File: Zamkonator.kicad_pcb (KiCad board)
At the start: 2 copper layers, 75 x 75 mm, 104 parts, among them J1 Screw_Terminal_01x06, J2 RJ45_Abracon_ARJP11A-MASA-B-A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, J3 Conn_01x08_Male, J4 Conn_02x08_Counter_Clockwise, K1 SRD-DC3V-SL-C, Q1 BCP56, T1 HR051142, U1 RTL8201F, U2 SI3404-A-GM, U3 EL3H7-G, U4 AN431, U5 MT2492, U6 ESP32-WROOM-32, U7 LTV-827S, U8 LTV-827S, X1 S3D50.000000B20F30T

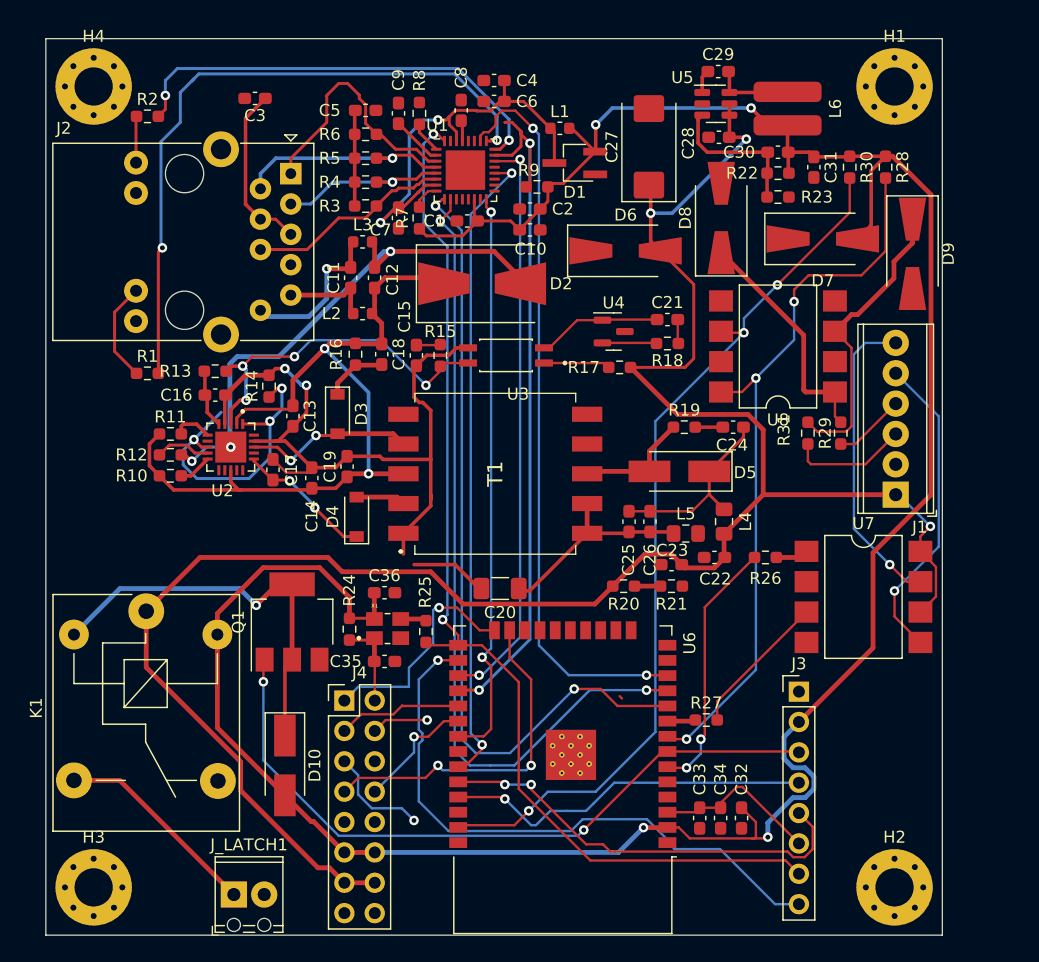
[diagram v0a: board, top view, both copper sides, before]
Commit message: Finish layout
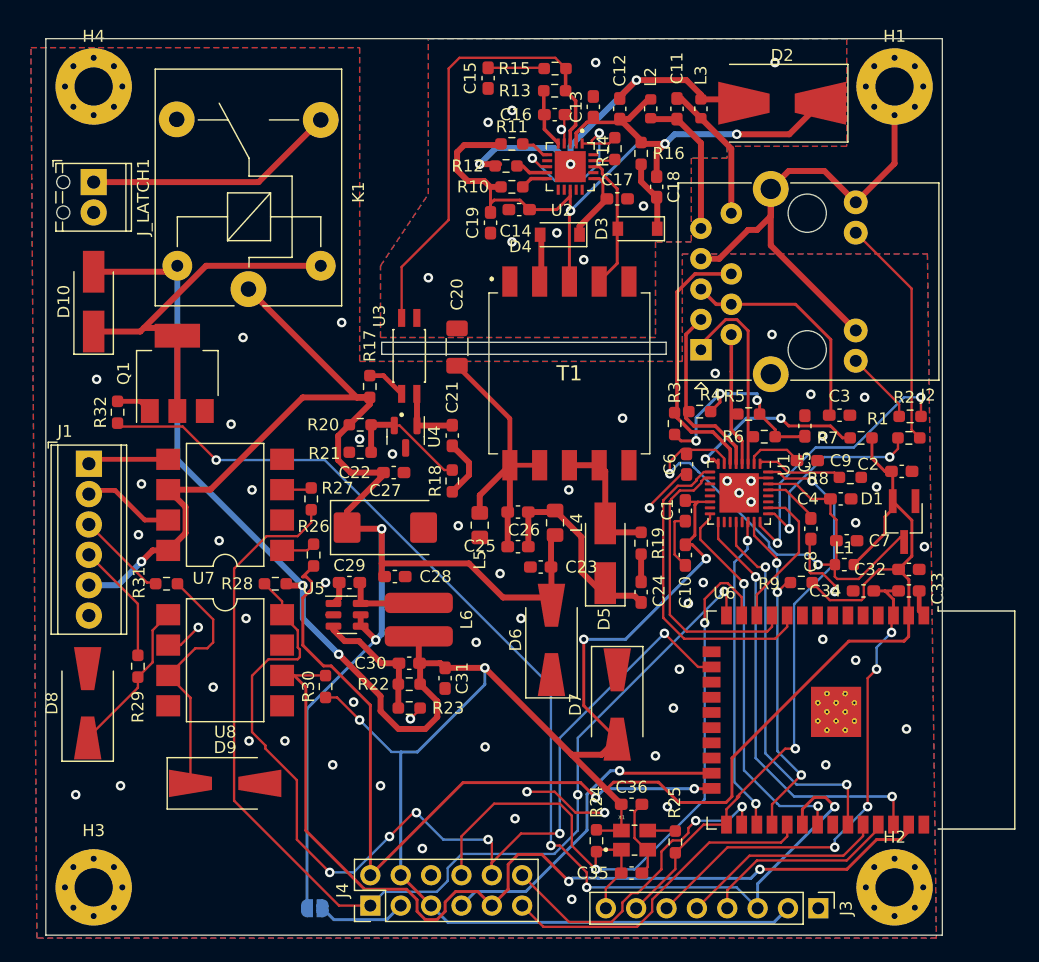
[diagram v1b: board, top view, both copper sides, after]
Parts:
- added JP1: SolderJumper_2_Open, Jumper:SolderJumper-2_P1.3mm_Open_RoundedPad1.0x1.5mm, B.Cu at (22.5, 72.8)
- added R32: R, Resistor_SMD:R_0603_1608Metric_Pad0.98x0.95mm_HandSolder, F.Cu at (6.00, 31.2)
- J4: value Conn_02x08_Counter_Clockwise -> Conn_02x06_Counter_Clockwise; footprint Connector_PinHeader_2.54mm:PinHeader_2x08_P2.54mm_Vertical -> Connector_PinHeader_2.54mm:PinHeader_2x06_P2.54mm_Vertical
- moved D9 72.6 mm to (15.0, 62.3), turned to 0 degrees
- moved R2 68.6 mm to (72.3, 31.6)
- moved J1 67.5 mm to (3.60, 35.6), turned to -90 degrees
- moved D8 66.8 mm to (3.50, 55.6)
- moved R1 63.9 mm to (72.2, 33.4), turned to 180 degrees
- moved R29 61.9 mm to (7.70, 52.5), turned to 90 degrees
- moved R28 61.8 mm to (19.2, 45.6), turned to 180 degrees
- moved R30 61.7 mm to (23.4, 54.2), turned to 90 degrees
- moved J_LATCH1 60.7 mm to (4.00, 12.0), turned to -90 degrees
- moved C3 55.6 mm to (66.4, 31.5), turned to 0 degrees
- moved R31 55.1 mm to (10.1, 45.6), turned to 180 degrees
- moved U7 54.0 mm to (15.0, 39.0), turned to 180 degrees
- moved U8 53.2 mm to (15.0, 52.0), turned to 0 degrees
- moved C29 52.7 mm to (25.4, 45.5)
- moved C30 52.7 mm to (30.4, 52.2)
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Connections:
- J1 pad 1: +12V -> /Wigand Intrerface/READER_LED
- J1 pad 2: GND -> /Wigand Intrerface/READER_BUZZER
- J1 pad 5: /Wigand Intrerface/READER_LED -> +12V
- J1 pad 6: /Wigand Intrerface/READER_BUZZER -> GND
- J3 pad 3: /ESP32/IO35 -> /ESP32/IO18
- J4 pad 1: /ESP32/IO2 -> /ESP32/IO12
- J4 pad 10: GND -> /ESP32/IO13
- J4 pad 11: +3.3V -> /ESP32/IO5
- J4 pad 12: +3.3V -> /ESP32/IO4
- J4 pad 2: /50MHZ CLOCK/CLK_EN -> /ESP32/IO2
- J4 pad 3: /ESP32/IO5 -> Net-(J4-Pad3)
- J4 pad 4: /ESP32/IO12 -> +3.3V
- J4 pad 5: /ESP32/IO13 -> +3.3V
- J4 pad 6: /ESP32/IO14 -> GND
- J4 pad 8: /ESP32/IO18 -> /50MHZ CLOCK/CLK_EN
- J4 pad 9: GND -> /ESP32/IO23
- Q1 pad 1: /ESP32/IO35 -> Net-(Q1-Pad1)
- R26 pad 1: /ESP32/IO34 -> /ESP32/IO2
- R27 pad 1: /ESP32/IO33 -> /ESP32/IO12
- R28 pad 2: /ESP32/IO32 -> /ESP32/IO13
- U6 pad 13: /ESP32/IO14 -> /50MHZ CLOCK/CLK_EN
- U6 pad 26: /50MHZ CLOCK/CLK_EN -> /ESP32/IO4
- U6 pad 6: /ESP32/IO34 -> unconnected-(U6-Pad6)
- U6 pad 7: /ESP32/IO35 -> unconnected-(U6-Pad7)
- U6 pad 8: /ESP32/IO32 -> unconnected-(U6-Pad8)
- U6 pad 9: /ESP32/IO33 -> unconnected-(U6-Pad9)
- U8 pad 8: /ESP32/IO32 -> /ESP32/IO13
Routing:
- net GND: track 0.00 -> 89.4 mm, vias 0 -> 58
- net /ESP32/IO12: track 4.76 -> 91.3 mm, vias 1 -> 2
- net /ESP32/IO18: track 10.2 -> 94.8 mm, vias 1 -> 4
- net /ESP32/IO13: track 8.83 -> 83.7 mm, vias 1 -> 6
- net VSS: track 66.2 -> 4.53 mm, vias 2 -> 10
- net /ESP32/IO32: track 61.5 -> 0.00 mm, vias 3 -> 0
- net /ESP32/IO35: track 58.8 -> 0.00 mm, vias 2 -> 0
- net /ESP32/EMAC_CRS_DV: track 62.0 -> 12.3 mm, vias 2 -> 0
- net /ESP32/EMAC_RXD1: track 67.9 -> 24.0 mm, vias 2 -> 0
- net /ESP32/IO2: track 19.1 -> 62.3 mm, vias 1 -> 2
- net +12V: track 172.7 -> 130.5 mm
- net +3.3V: track 218.6 -> 260.5 mm, vias 4 -> 6
- net /50MHZ CLOCK/CLK_OUT: track 90.3 -> 49.5 mm
- net /ESP32/EMAC_RXD0: track 67.4 -> 27.2 mm, vias 2 -> 0
- net Net-(R1-Pad2): track 56.0 -> 16.9 mm
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- added copper zone on B.Cu, net GND
- added copper zone on F.Cu, net GND
- added copper zone on B.Cu, net VSS
- added copper zone on F.Cu, net VSS
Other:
- outline, holes or cut-outs redrawn
